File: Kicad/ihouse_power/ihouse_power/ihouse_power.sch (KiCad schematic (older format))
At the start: 29 parts, among them J10 Conn_02x07_Odd_Even, J11 Conn_01x14, J19 I2C, J21 RS232, J22 Nextion, J30 OPT3, J5 Conn_01x16, J500 OPTIC, J502 LEAK1, J503 LEAK2, J504 LEAK3, J505 DHT22, J506 Valve1, J507 Conn_01x14, J508 Valve1, J509 Valve2, J510 Valve2, J511 OPT2, J512 OPT1, J6 Conn_01x06, J7 Conn_02x07_Odd_Even, J8 Conn_01x16, J9 Conn_01x06, U12 MAX232

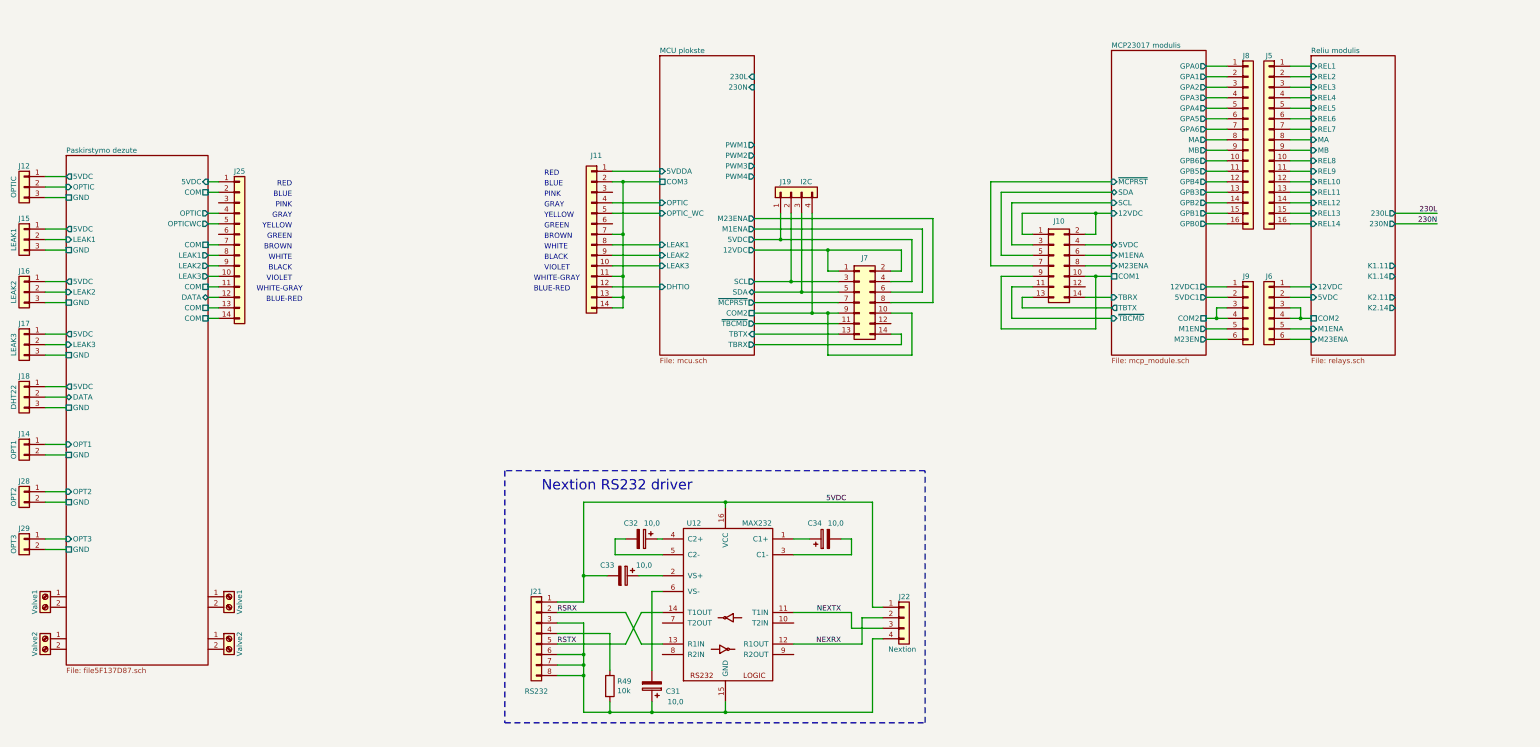
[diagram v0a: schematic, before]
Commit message: schemos ir pcb ruosimas
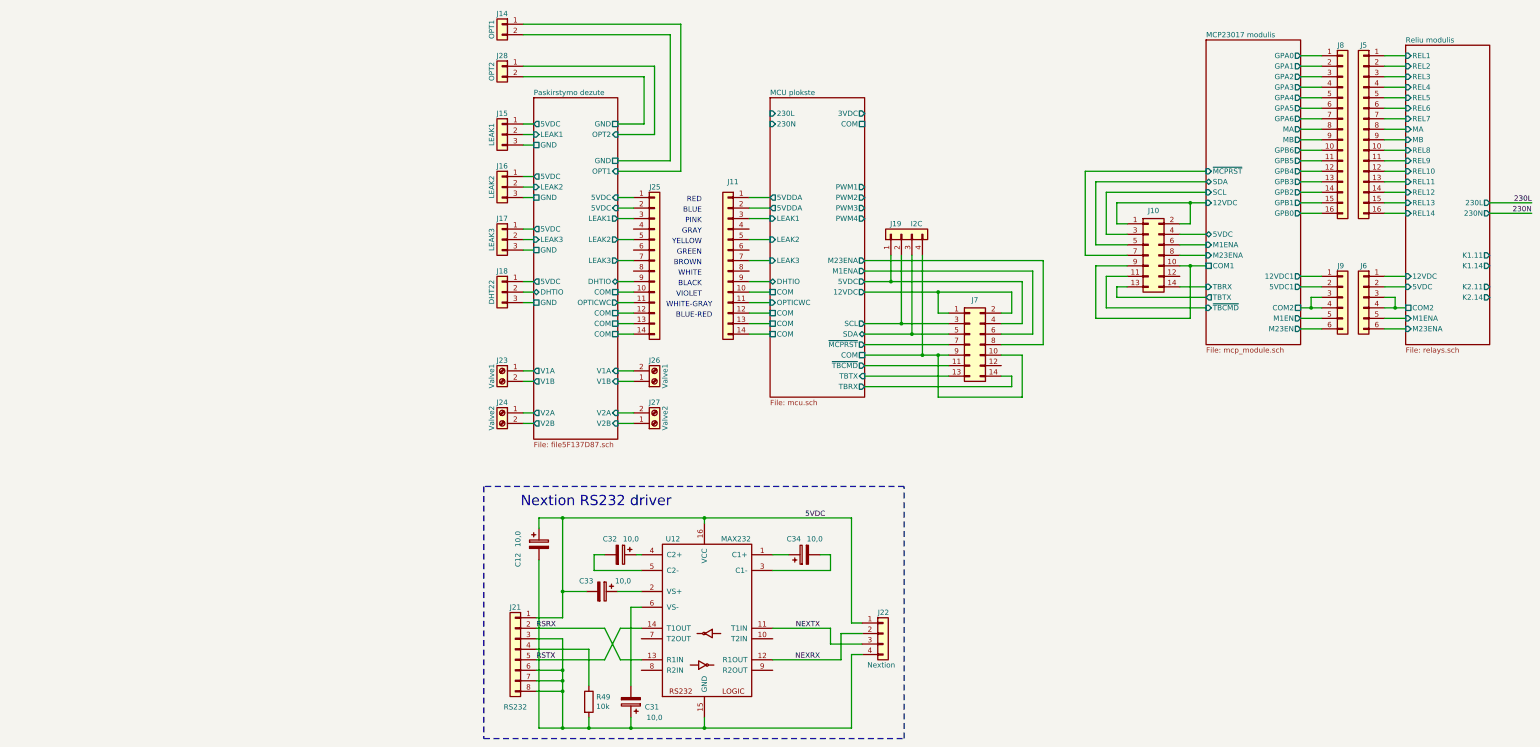
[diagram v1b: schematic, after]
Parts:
- removed J30: OPT3, symbol Connector_Generic:Conn_01x02
- removed J500: OPTIC, symbol Connector_Generic:Conn_01x03
- added C12: 10,0, Capacitor_SMD:CP_Elec_3x5.4, symbol Device:CP
- J14: renamed from J512; footprint (none) -> Connector_JST:JST_EH_B2B-EH-A_1x02_P2.50mm_Vertical
- J15: renamed from J502; footprint (none) -> Connector_JST:JST_EH_B3B-EH-A_1x03_P2.50mm_Vertical
- J16: renamed from J503; footprint (none) -> Connector_JST:JST_EH_B3B-EH-A_1x03_P2.50mm_Vertical
- J17: renamed from J504; footprint (none) -> Connector_JST:JST_EH_B3B-EH-A_1x03_P2.50mm_Vertical
- J18: renamed from J505; footprint (none) -> Connector_JST:JST_EH_B3B-EH-A_1x03_P2.50mm_Vertical
- J23: renamed from J506; footprint (none) -> TerminalBlock_4Ucon:TerminalBlock_4Ucon_1x02_P3.50mm_Horizontal
- J24: renamed from J510; footprint (none) -> TerminalBlock_4Ucon:TerminalBlock_4Ucon_1x02_P3.50mm_Horizontal
- J25: renamed from J507; footprint (none) -> Connector_Multicomp:Multicomp_MC9A12-1434_2x07_P2.54mm_Vertical
- J26: renamed from J508; footprint (none) -> TerminalBlock_4Ucon:TerminalBlock_4Ucon_1x02_P3.50mm_Horizontal
- J27: renamed from J509; footprint (none) -> TerminalBlock_4Ucon:TerminalBlock_4Ucon_1x02_P3.50mm_Horizontal
- J28: renamed from J511; footprint (none) -> Connector_JST:JST_EH_B2B-EH-A_1x02_P2.50mm_Vertical
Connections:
- net MCU plokste/OPTIC_WC is gone; now on net MCU plokste/LEAK2: J11.5 (Pin_5)
- net Paskirstymo dezute/5VDC is gone; now on net Paskirstymo dezute/5VDC: J18.1 (Pin_1)
- net Paskirstymo dezute/COM is gone; now on net Paskirstymo dezute/COM: J25.14 (Pin_14)
- net Paskirstymo dezute/GND is gone; now on net Paskirstymo dezute/GND: J18.3 (Pin_3)
- net Paskirstymo dezute/LEAK1 is gone; now on net Paskirstymo dezute/LEAK1: J15.2 (Pin_2)
- net Paskirstymo dezute/LEAK2 is gone; now on net Paskirstymo dezute/LEAK2: J16.2 (Pin_2)
- net Paskirstymo dezute/LEAK3 is gone; now on net Paskirstymo dezute/LEAK3: J17.2 (Pin_2)
- net 5VDC: now also C12.1
- net MCU plokste/5VDDA: now also J11.2 (Pin_2); no longer J11.1 (Pin_1)
- net MCU plokste/DHTIO: now also J11.9 (Pin_9); no longer J11.12 (Pin_12)
- net MCU plokste/LEAK1: now also J11.3 (Pin_3); no longer J11.8 (Pin_8)
- net MCU plokste/LEAK2: no longer J11.9 (Pin_9)
- net MCU plokste/LEAK3: now also J11.7 (Pin_7); no longer J11.10 (Pin_10)
- net Paskirstymo dezute/5VDC: no longer J25.1 (Pin_1)
- net Paskirstymo dezute/COM: no longer J25.11 (Pin_11)
- net Paskirstymo dezute/GND: no longer J14.2 (Pin_2)
- net Paskirstymo dezute/LEAK1: no longer J25.8 (Pin_8)
- net Paskirstymo dezute/LEAK2: no longer J25.9 (Pin_9)
- net Paskirstymo dezute/LEAK3: no longer J25.10 (Pin_10)
- net Paskirstymo dezute/OPTICWC: now also J25.11 (Pin_11); no longer J25.5 (Pin_5)
- net at C31.1, J21.3 (Pin_3), J21.6 (Pin_6)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: now also C12.2
- net Paskirstymo dezute/LEAK1: now reaches J25.3 (Pin_3)
- net Paskirstymo dezute/V1A: now reaches J23.1 (Pin_1)
- net Paskirstymo dezute/V1B: now reaches J23.2 (Pin_2)
- net Paskirstymo dezute/V2A: now reaches J24.1 (Pin_1)
- net Paskirstymo dezute/V2B: now reaches J24.2 (Pin_2)
- net Paskirstymo dezute/V1B: now reaches J26.1 (Pin_1)
- net Paskirstymo dezute/V1A: now reaches J26.2 (Pin_2)
- net Paskirstymo dezute/V2B: now reaches J27.1 (Pin_1)
- net Paskirstymo dezute/V2A: now reaches J27.2 (Pin_2)
- net MCU plokste/COM2 renamed MCU plokste/COM
- removed net MCU plokste/COM3: J11.11 (Pin_11), J11.13 (Pin_13), J11.14 (Pin_14), J11.2 (Pin_2), J11.7 (Pin_7)
- net MCU plokste/OPTIC: no longer names the net of J11.4 (Pin_4)
- net Paskirstymo dezute/COM renamed Paskirstymo dezute/5VDC
- net Paskirstymo dezute/COM renamed Paskirstymo dezute/LEAK3
- net Paskirstymo dezute/DATA renamed Paskirstymo dezute/COM
- net Paskirstymo dezute/DATA renamed Paskirstymo dezute/DHTIO
- net Paskirstymo dezute/OPTIC: no longer names the net of J25.4 (Pin_4)
- new net MCU plokste/5VDDA: J11.1 (Pin_1)
- new net MCU plokste/COM: J11.10 (Pin_10)
- new net MCU plokste/COM: J11.12 (Pin_12)
- new net MCU plokste/COM: J11.13 (Pin_13)
- new net MCU plokste/COM: J11.14 (Pin_14)
- new net MCU plokste/OPTICWC: J11.11 (Pin_11)
- new net Paskirstymo dezute/5VDC: J25.1 (Pin_1)
- new net Paskirstymo dezute/COM: J25.10 (Pin_10)
- new net Paskirstymo dezute/DHTIO: J25.9 (Pin_9)
- new net Paskirstymo dezute/GND: J14.2 (Pin_2)
- new net Paskirstymo dezute/LEAK2: J25.5 (Pin_5)
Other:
- moved on the sheet: C31, C32, C33, C34, J10, J11, J19, J21, J22, J5, J6, J7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
